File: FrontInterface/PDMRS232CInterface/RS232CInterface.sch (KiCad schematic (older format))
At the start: 37 parts, among them IC1 ADM3251EARWZ, J1 Screw_Terminal_01x02, J2 DB9_Female, J4 Conn_01x04, Q1 2N7000, Q2 2N7000, U1 MCP2561-E-SN, U2 MCP16301, U3 BluePill_STM32F103C

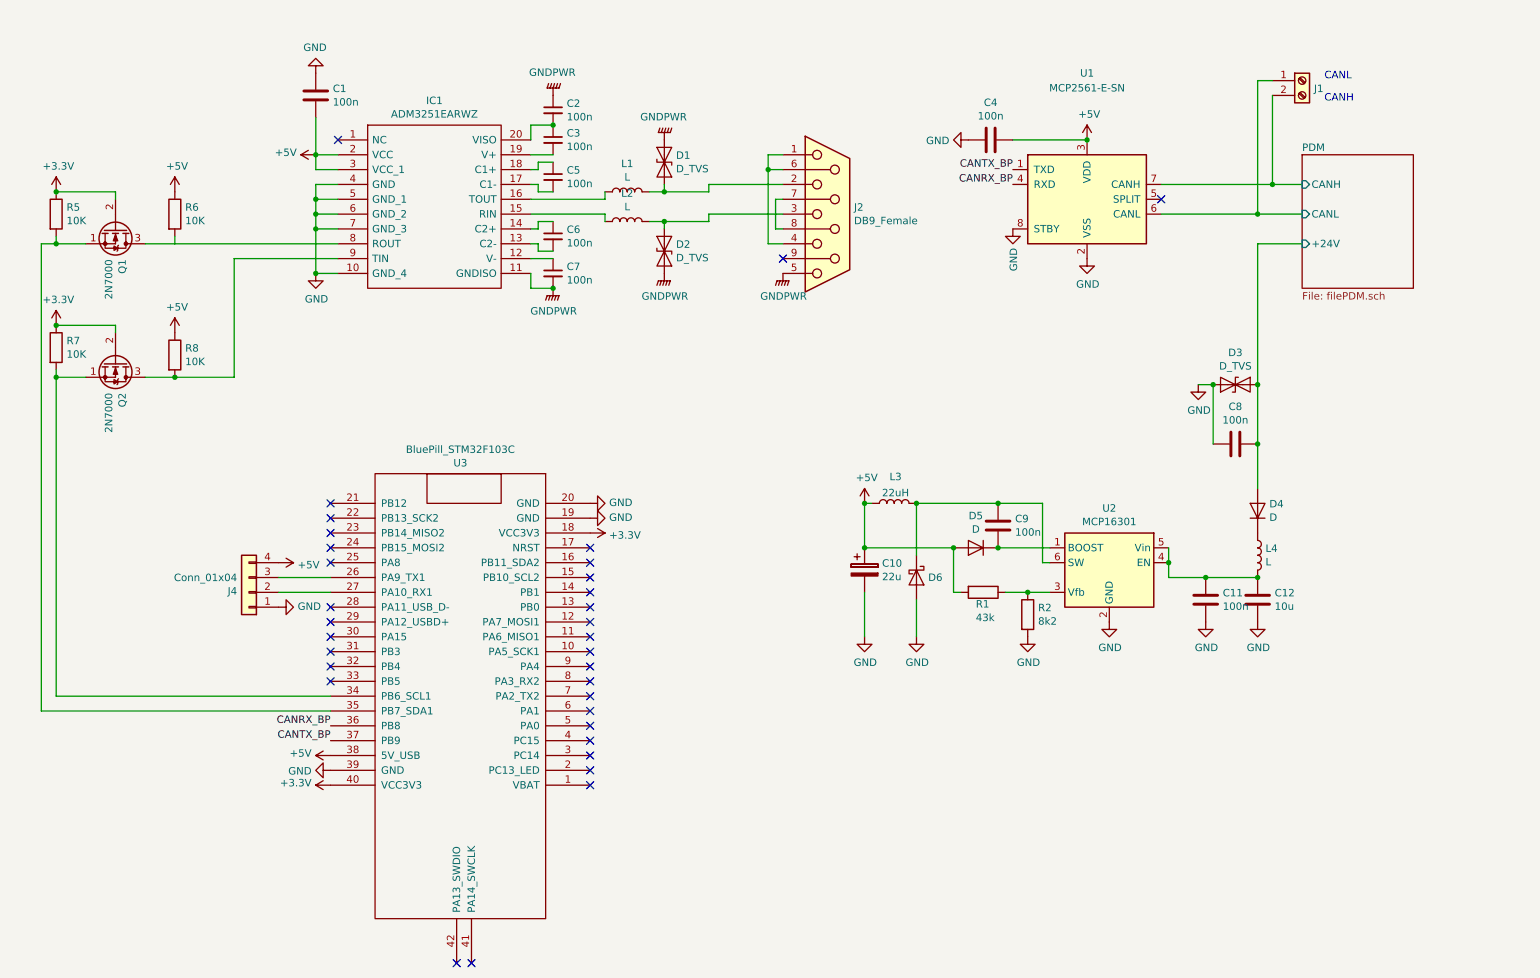
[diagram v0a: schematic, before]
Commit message: PCB updated
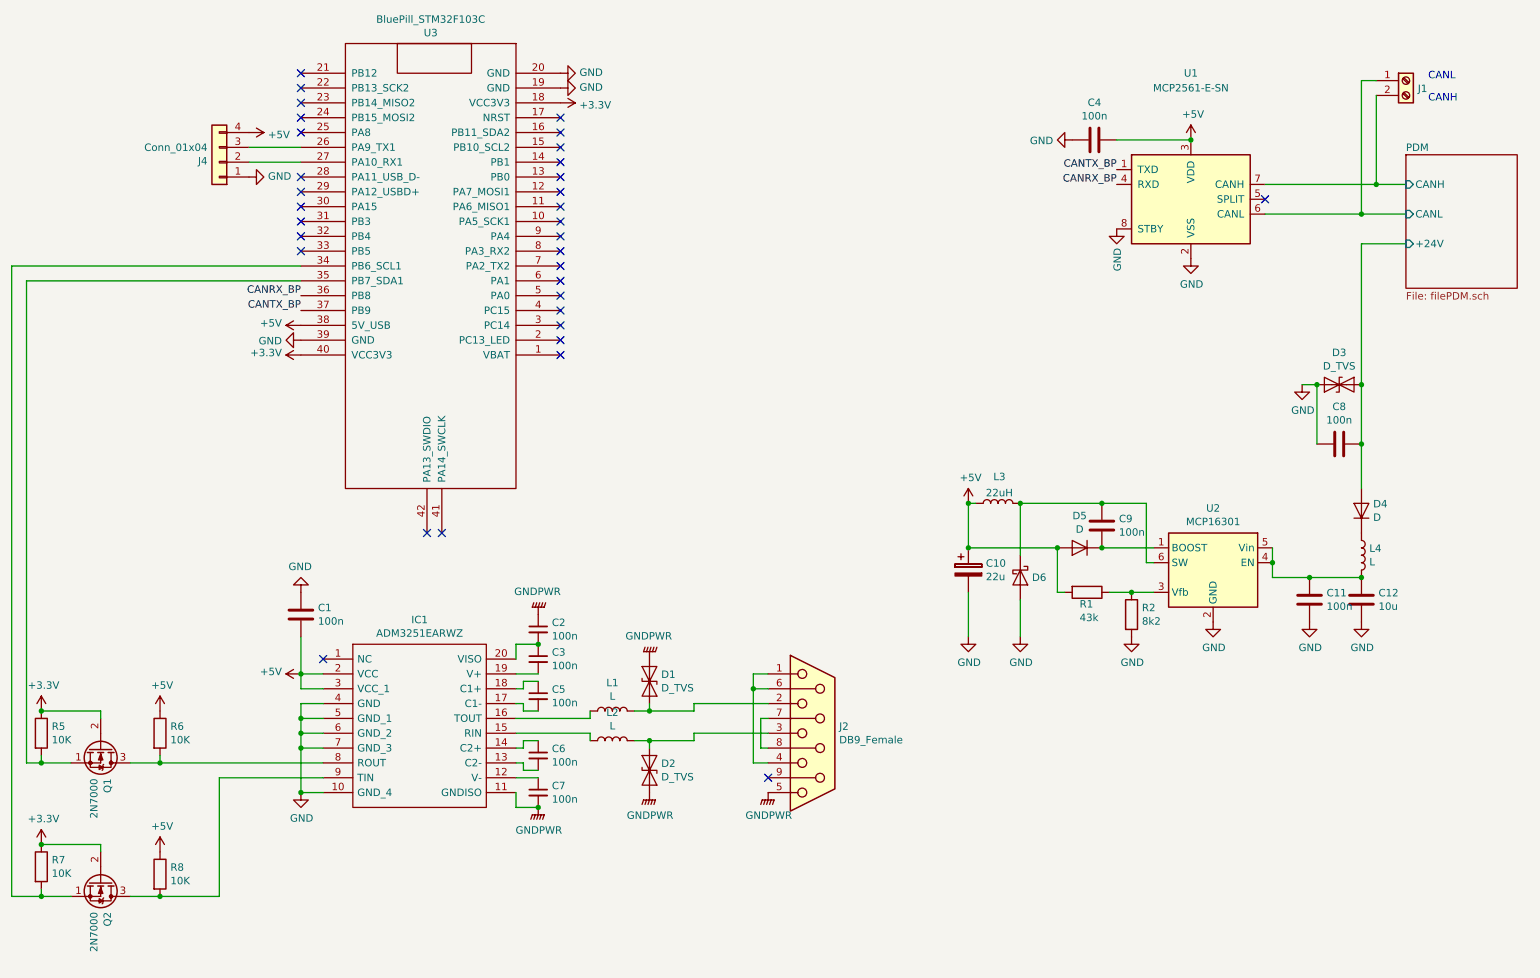
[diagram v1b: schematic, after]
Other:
- moved on the sheet: C1, C10, C11, C12, C2, C3, C4, C5, C6, C7, C8, C9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
